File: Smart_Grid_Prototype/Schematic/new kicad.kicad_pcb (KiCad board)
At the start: 2 copper layers, 144.8 x 116.8 mm, 70 parts, among them J1 EXT_POW, J2 24VAC _LOAD, J3 AC_INPUT, J4 DC_LOAD, J5 POW_SHARE, Q1 BD139, Q2 BD139, Q3 BD139, Q4 BD139, Q5 BD139, Q6 BD139, Q7 BD139, U1 ESP8266, U10 PC817, U11 PC817, U12 PC817, U13 PC817, U14 PC817, U15 PC817, U16 PC817, U2 RELAY_INT, U3 RELAY_PS, U4 PC817, U5 LM7824_TO220, U6 PC817, U7 PC817, U8 LM317_TO-220, U9 PC817

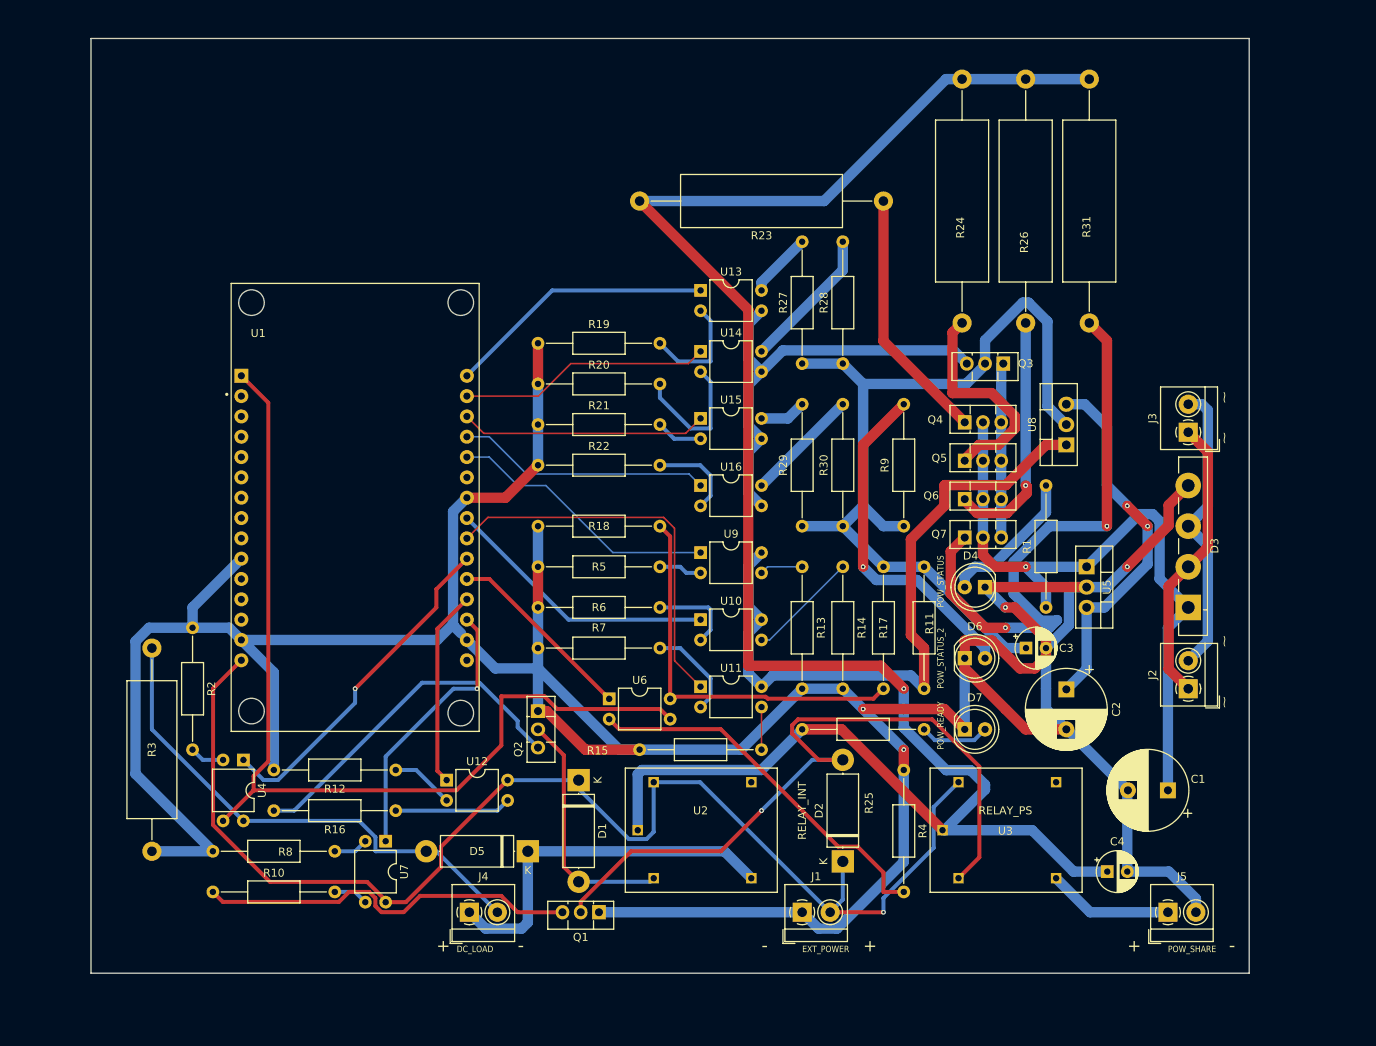
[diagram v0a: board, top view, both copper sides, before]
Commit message: Perfect PCB
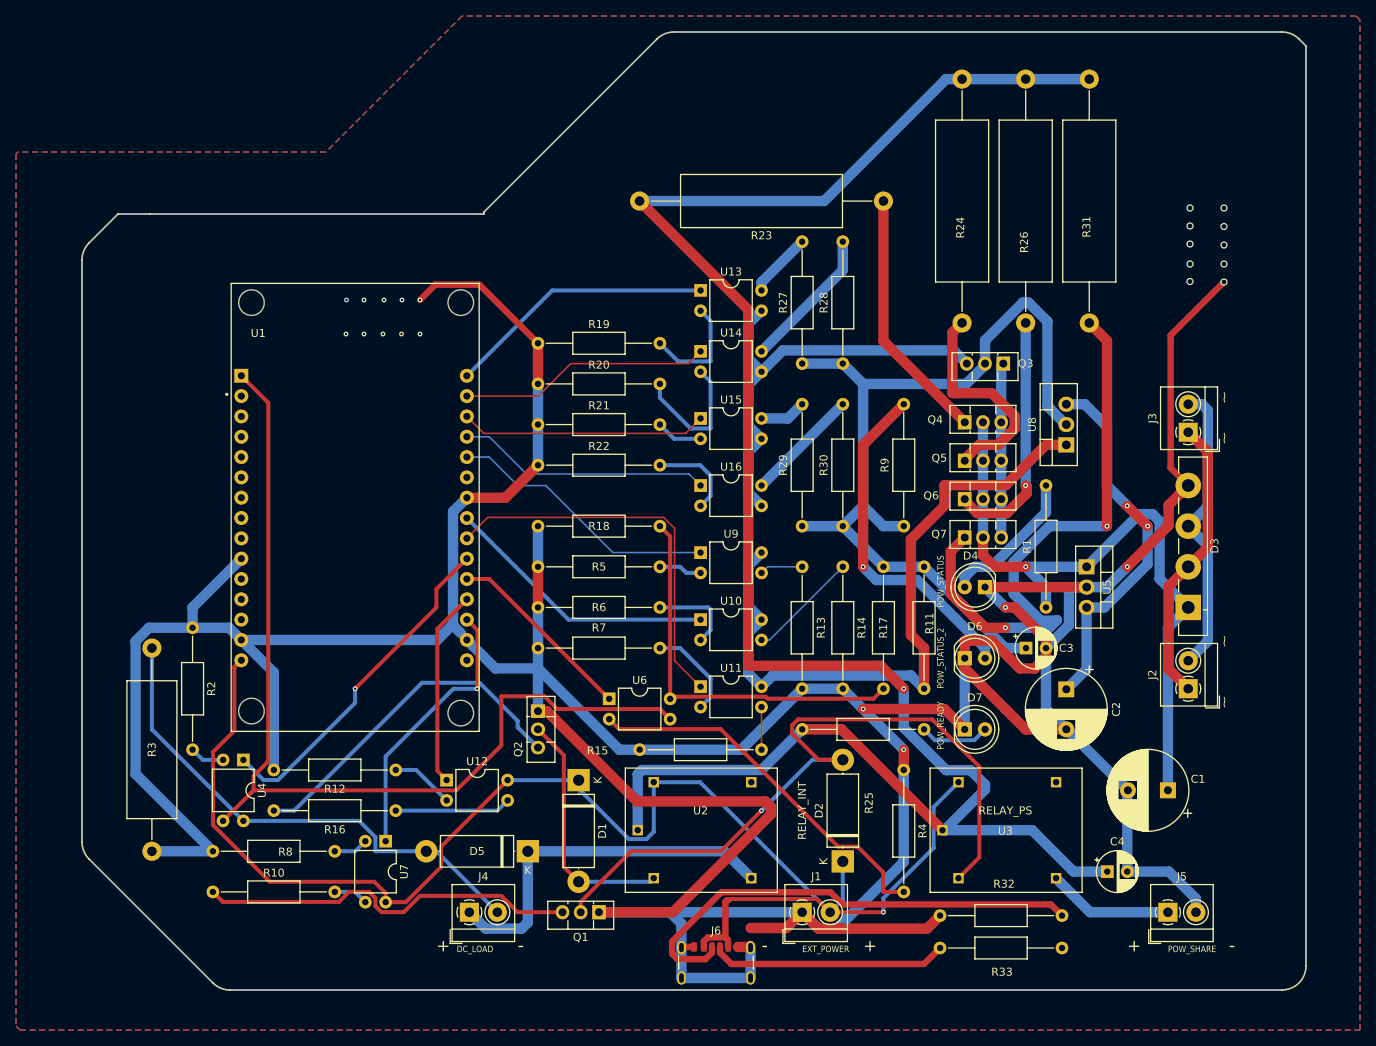
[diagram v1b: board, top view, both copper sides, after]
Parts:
- added J6: USB_C_Receptacle_PowerOnly_6P, Connector_USB:USB_C_Receptacle_GCT_USB4125-xx-x-0190_6P_TopMnt_Horizontal, F.Cu at (149.2, 152.2)
- added R32: 5.1k, Resistor_THT:R_Axial_DIN0207_L6.3mm_D2.5mm_P15.24mm_Horizontal, F.Cu at (177.3, 145.2)
- added R33: 5.1k, Resistor_THT:R_Axial_DIN0207_L6.3mm_D2.5mm_P15.24mm_Horizontal, F.Cu at (177.3, 149.2)
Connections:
- net /EXT_POWER renamed VCC
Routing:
- net GND: track 467.4 -> 612.4 mm, vias 4 -> 24
- net Net-(J6-CC1): track 0.00 -> 60.3 mm
- net Net-(J6-CC2): track 0.00 -> 29.6 mm
- net VCC: track 161.9 -> 185.7 mm
- added copper zone on B.Cu, net GND
- added copper zone on F.Cu, net GND
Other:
- board size 144.8 x 116.8 mm -> 153 x 119.8 mm
